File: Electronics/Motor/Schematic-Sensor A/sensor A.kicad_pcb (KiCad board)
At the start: 2 copper layers, 12 x 27 mm, 3 parts, among them J1 CONN_01X06, U1 MA700

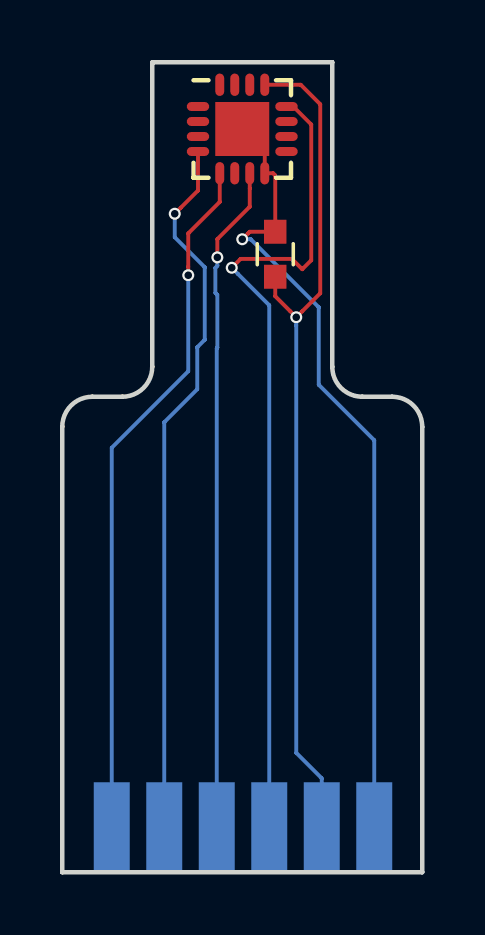
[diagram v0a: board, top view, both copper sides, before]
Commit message: current work
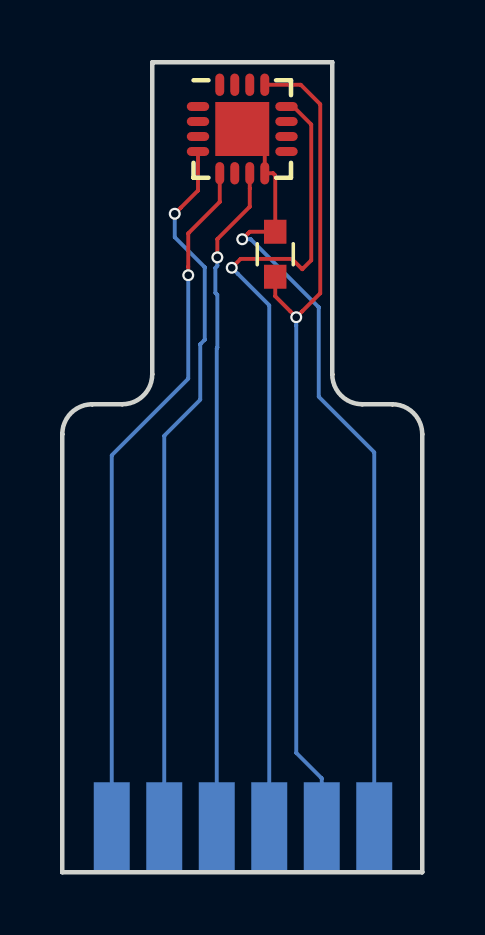
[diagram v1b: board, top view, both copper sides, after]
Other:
- outline, holes or cut-outs redrawn
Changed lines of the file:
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@@
     (links 12)
     (no_connects 0)
-    (area 85.336667 58.895 99.075001 89.755)
+    (area 85.336667 58.47 99.075001 89.755)
     (thickness 1.6)
     (drawings 12)
@@
     (pad_to_mask_clearance 0.2)
     (aux_axis_origin 0 0)
-    (visible_elements 7FFFFFFF)
+    (visible_elements 7FFFEFFF)
     (pcbplotparams
       (layerselection 0x010c0_80000001)
@@
     )
   )
-  (gr_arc (start 98 72.15) (end 98 71.15) (angle 90) (layer Edge.Cuts) (width 0.15))
-  (gr_arc (start 97 70.15) (end 97 71.15) (angle 90) (layer Edge.Cuts) (width 0.15))
-  (gr_arc (start 88 72.15) (end 87 72.15) (angle 90) (layer Edge.Cuts) (width 0.15))
-  (gr_arc (start 89 70.15) (end 90 70.15) (angle 90) (layer Edge.Cuts) (width 0.15))
-  (gr_line (start 98 71.15) (end 97 71.15) (layer Edge.Cuts) (width 0.15))
-  (gr_line (start 99 87) (end 99 72.15) (layer Edge.Cuts) (width 0.15))
-  (gr_line (start 88 71.15) (end 89 71.15) (layer Edge.Cuts) (width 0.15))
-  (gr_line (start 87 87) (end 87 72.15) (layer Edge.Cuts) (width 0.15))
+  (gr_arc (start 98 72.4) (end 98 71.4) (angle 90) (layer Edge.Cuts) (width 0.15))
+  (gr_arc (start 97 70.4) (end 97 71.4) (angle 90) (layer Edge.Cuts) (width 0.15))
+  (gr_arc (start 88 72.4) (end 87 72.4) (angle 90) (layer Edge.Cuts) (width 0.15))
+  (gr_arc (start 89 70.4) (end 90 70.4) (angle 90) (layer Edge.Cuts) (width 0.15))
+  (gr_line (start 98 71.4) (end 97 71.4) (layer Edge.Cuts) (width 0.15))
+  (gr_line (start 99 87) (end 99 72.4) (layer Edge.Cuts) (width 0.15))
+  (gr_line (start 88 71.4) (end 89 71.4) (layer Edge.Cuts) (width 0.15))
+  (gr_line (start 87 87) (end 87 72.4) (layer Edge.Cuts) (width 0.15))
   (gr_line (start 87 87) (end 99 87) (layer Edge.Cuts) (width 0.15))
   (gr_line (start 90 60) (end 96 60) (layer Edge.Cuts) (width 0.15))
-  (gr_line (start 96 60) (end 96 70.15) (layer Edge.Cuts) (width 0.15))
-  (gr_line (start 90 60) (end 90 70.15) (layer Edge.Cuts) (width 0.15))
+  (gr_line (start 96 60) (end 96 70.4) (layer Edge.Cuts) (width 0.15))
+  (gr_line (start 90 60) (end 90 70.4) (layer Edge.Cuts) (width 0.15))
   (segment (start 94.999999 68.300001) (end 94.8 68.5) (width 0.13) (layer F.Cu) (net 1))
   (segment (start 95.6 61.4) (end 95.6 67.7) (width 0.13) (layer F.Cu) (net 1))
@@
   (segment (start 94.8 83.02) (end 94.8 68.782842) (width 0.13) (layer B.Cu) (net 1))
   (via (at 94.8 68.5) (size 0.4) (drill 0.25) (layers F.Cu B.Cu) (net 1))
-  (segment (start 97.4 72.6) (end 95.55 70.75) (width 0.13) (layer B.Cu) (net 2))
-  (segment (start 97.4 85.5) (end 97.4 72.6) (width 0.13) (layer B.Cu) (net 2))
-  (segment (start 95.55 70.75) (end 95.55 68.167164) (width 0.13) (layer B.Cu) (net 2))
+  (segment (start 97.4 85.5) (end 97.4 73) (width 0.13) (layer B.Cu) (net 2))
+  (segment (start 97.4 73) (end 95.55 71.15) (width 0.13) (layer B.Cu) (net 2))
+  (segment (start 95.55 71.15) (end 95.55 68.167164) (width 0.13) (layer B.Cu) (net 2))
   (segment (start 95.55 68.167164) (end 93.282842 65.900006) (width 0.13) (layer B.Cu) (net 2))
   (segment (start 93.282842 65.900006) (end 93 65.900006) (width 0.13) (layer B.Cu) (net 2))
@@
   (segment (start 94.1 63.77) (end 94.03 63.7) (width 0.13) (layer F.Cu) (net 2))
   (segment (start 94.03 63.7) (end 93.75 63.7) (width 0.13) (layer F.Cu) (net 2))
-  (segment (start 91.2 67.1) (end 91.2 70.3) (width 0.13) (layer B.Cu) (net 3))
-  (segment (start 91.2 70.3) (end 88.65 72.85) (width 0.13) (layer B.Cu) (net 3))
-  (segment (start 88.65 72.85) (end 88.65 85.5) (width 0.13) (layer B.Cu) (net 3))
+  (segment (start 91.2 67.1) (end 91.2 70.55) (width 0.13) (layer B.Cu) (net 3))
+  (segment (start 91.2 70.55) (end 88.65 73.1) (width 0.13) (layer B.Cu) (net 3))
+  (segment (start 88.65 73.1) (end 88.65 85.5) (width 0.13) (layer B.Cu) (net 3))
   (segment (start 91.2 66.817158) (end 91.2 67.1) (width 0.13) (layer F.Cu) (net 3))
   (segment (start 91.2 65.705) (end 91.2 66.817158) (width 0.13) (layer F.Cu) (net 3))
@@
   (segment (start 90.75 65.832842) (end 91.75 66.832842) (width 0.13) (layer B.Cu) (net 4))
   (segment (start 91.75 66.832842) (end 91.75 69.25) (width 0.13) (layer B.Cu) (net 4))
-  (segment (start 91.75 69.25) (end 91.5 69.5) (width 0.13) (layer B.Cu) (net 4))
-  (segment (start 91.5 69.5) (end 91.5 70.9) (width 0.13) (layer B.Cu) (net 4))
-  (segment (start 91.5 70.9) (end 90.4 72) (width 0.13) (layer B.Cu) (net 4))
-  (segment (start 90.4 72) (end 90.4 85.5) (width 0.13) (layer B.Cu) (net 4))
+  (segment (start 91.75 69.25) (end 91.6 69.4) (width 0.13) (layer B.Cu) (net 4))
+  (segment (start 91.6 69.4) (end 91.6 71.25) (width 0.13) (layer B.Cu) (net 4))
+  (segment (start 91.6 71.25) (end 90.4 72.45) (width 0.13) (layer B.Cu) (net 4))
+  (segment (start 90.4 72.45) (end 90.4 85.5) (width 0.13) (layer B.Cu) (net 4))
   (segment (start 90.949999 64.850001) (end 90.75 65.05) (width 0.13) (layer F.Cu) (net 4))
   (segment (start 91.525 62.975) (end 91.525 64.275) (width 0.13) (layer F.Cu) (net 4))
